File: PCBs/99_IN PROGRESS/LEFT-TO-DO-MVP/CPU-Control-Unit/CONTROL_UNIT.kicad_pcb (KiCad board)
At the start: 2 copper layers, 120.6 x 59.2 mm, 16 parts, among them U1 PLCC32_28_28C256, U10 74LS08, U11 74LS08, U12 74LS139, U13 74LS154, U14 74LS08, U15 74HC245, U16 74HC245, U2 74HC245, U3 74HC245, U4 PLCC32_28_28C256, U5 74LS139, U6 74LS154, U7 74LS154, U8 74LS04, U9 74LS08

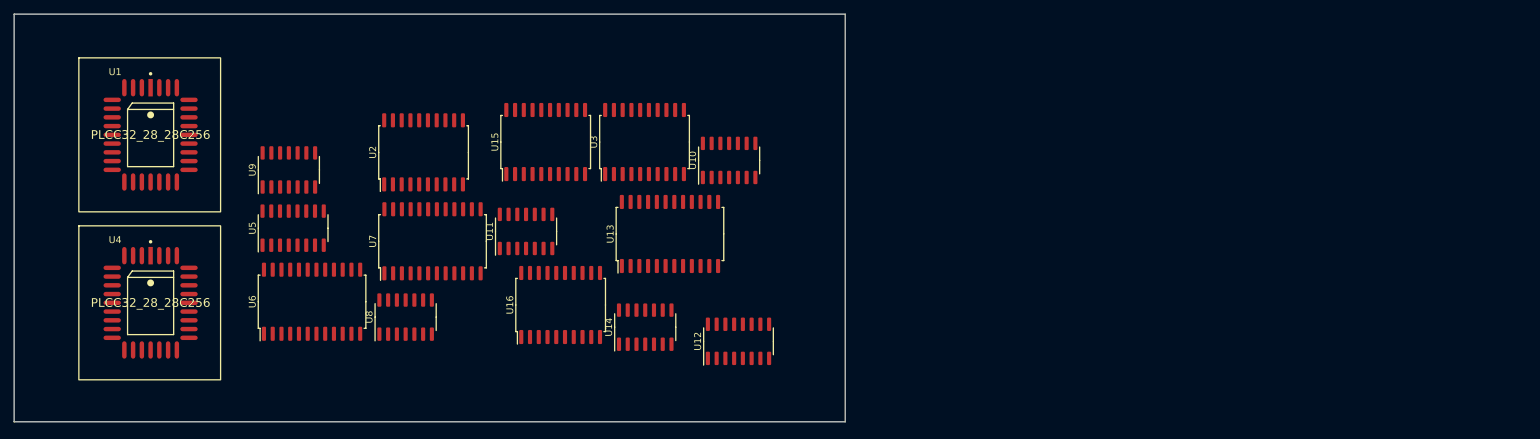
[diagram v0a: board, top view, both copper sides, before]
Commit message: saving
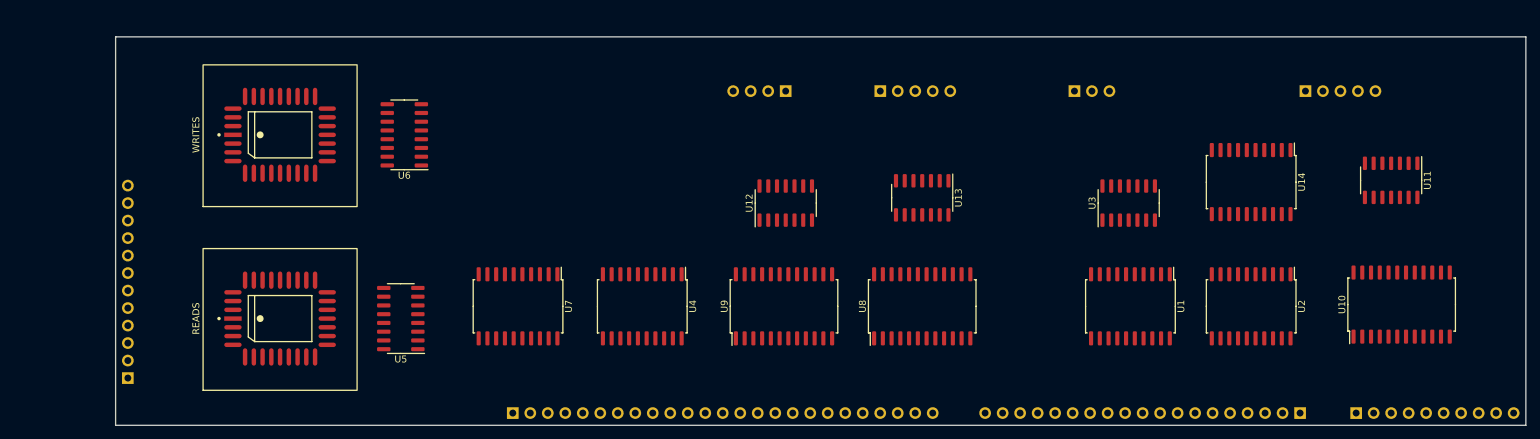
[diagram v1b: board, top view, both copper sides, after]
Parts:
- added J1: Conn_01x05, Connector_PinHeader_2.54mm:PinHeader_1x05_P2.54mm_Vertical, B.Cu at (224.3, 68.3)
- added J2: Conn_01x12, Connector_PinHeader_2.54mm:PinHeader_1x12_P2.54mm_Vertical, B.Cu at (53.3, 110.0)
- added J3: Conn_01x03, Connector_PinHeader_2.54mm:PinHeader_1x03_P2.54mm_Vertical, B.Cu at (190.8, 68.3)
- added J4: Conn_01x05, Connector_PinHeader_2.54mm:PinHeader_1x05_P2.54mm_Vertical, B.Cu at (162.6, 68.3)
- added J5: Conn_01x25, Connector_PinHeader_2.54mm:PinHeader_1x25_P2.54mm_Vertical, B.Cu at (109.2, 115.1)
- added J6: Conn_01x19, Connector_PinHeader_2.54mm:PinHeader_1x19_P2.54mm_Vertical, B.Cu at (223.5, 115.1)
- added J7: Conn_01x04, Connector_PinHeader_2.54mm:PinHeader_1x04_P2.54mm_Vertical, B.Cu at (148.8, 68.3)
- added J8: Conn_01x10, Connector_PinHeader_2.54mm:PinHeader_1x10_P2.54mm_Vertical, B.Cu at (231.6, 115.1)
- U1, U4: value PLCC32_28_28C256 -> 74HC245; footprint Stephenv6:PLCC-32-SOCKET-Microchip-32J-10_2001-B-IPC_A -> Package_SO:SOIC-20W_7.5x12.8mm_P1.27mm
- U10, U9: value 74LS08 -> 74LS154; footprint Package_SO:SOIC-14_3.9x8.7mm_P1.27mm -> Package_SO:SOIC-24W_7.5x15.4mm_P1.27mm
- U12: value 74LS139 -> 74LS08; footprint Package_SO:SOIC-16_3.9x9.9mm_P1.27mm -> Package_SO:SOIC-14_3.9x8.7mm_P1.27mm
- U13: value 74LS154 -> 74LS08; footprint Package_SO:SOIC-24W_7.5x15.4mm_P1.27mm -> Package_SO:SOIC-14_3.9x8.7mm_P1.27mm
- U14: value 74LS08 -> 74HC245; footprint Package_SO:SOIC-14_3.9x8.7mm_P1.27mm -> Package_SO:SOIC-20W_7.5x12.8mm_P1.27mm
- U15, U16: value 74HC245 -> PLCC32_28_28C256; footprint Package_SO:SOIC-20W_7.5x12.8mm_P1.27mm -> LIBRARY-8-bit-computer:Socket-PLCC-32
- U3: value 74HC245 -> 74LS08; footprint Package_SO:SOIC-20W_7.5x12.8mm_P1.27mm -> Package_SO:SOIC-14_3.9x8.7mm_P1.27mm
- U6: value 74LS154 -> 74LS138; footprint Package_SO:SOIC-24W_7.5x15.4mm_P1.27mm -> Package_SO:SOIC-16_3.9x9.9mm_P1.27mm
- U7: value 74LS154 -> 74HC245; footprint Package_SO:SOIC-24W_7.5x15.4mm_P1.27mm -> Package_SO:SOIC-20W_7.5x12.8mm_P1.27mm
- U8: value 74LS04 -> 74LS154; footprint Package_SO:SOIC-14_3.9x8.7mm_P1.27mm -> Package_SO:SOIC-24W_7.5x15.4mm_P1.27mm
- moved U1 144.4 mm to (198.9, 99.6), turned to -90 degrees
- moved U11 125.8 mm to (236.7, 81.3), turned to -90 degrees
- moved U2 122.2 mm to (216.4, 99.6), turned to -90 degrees
- moved U10 99.8 mm to (238.3, 99.3)
- moved U14 90.4 mm to (216.4, 81.5), turned to -90 degrees
- moved U8 75.0 mm to (168.7, 99.6)
- moved U9 74.6 mm to (148.6, 99.6)
- moved U4 71.4 mm to (128.0, 99.6), turned to -90 degrees
- moved U3 70.8 mm to (198.6, 84.6)
- moved U16 47.6 mm to (75.4, 74.7)
- moved U15 46.3 mm to (75.4, 101.3)
- moved U13 37.0 mm to (168.7, 83.8), turned to -90 degrees
- moved U6 27.7 mm to (93.5, 74.7), turned to 180 degrees
- moved U12 21.2 mm to (148.8, 84.6)
- moved U5 20.4 mm to (93.0, 101.3), turned to 180 degrees
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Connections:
- net ~{EN_WRITE_0} renamed ~{EN_READ_GPR}
- U1 pad 1: unconnected-(U1-Pad1) -> VCC
- U1 pad 10: STEP1 -> GND
- U1 pad 11: STEP0 -> unconnected-(U1-Pad11)
- U1 pad 13: WRITE0 -> unconnected-(U1-Pad13)
- U1 pad 14: WRITE1 -> unconnected-(U1-Pad14)
- U1 pad 15: WRITE2 -> unconnected-(U1-Pad15)
- U1 pad 16: GND -> GPR2
- U1 pad 17: unconnected-(U1-Pad17) -> GPR1
- U1 pad 18: WRITE3 -> GPR0
- U1 pad 19: WRITE4 -> ~{EN_WRITE_GPR}
- U1 pad 2: GND -> μ2_0
- U1 pad 20: WRITE5 -> VCC
- U1 pad 3: GND -> μ2_1
- U1 pad 4: INSTRUCTION3 -> μ2_2
- U1 pad 5: INSTRUCTION2 -> GND
- U1 pad 6: INSTRUCTION1 -> GND
- U1 pad 7: INSTRUCTION0 -> GND
- U1 pad 8: STEP3 -> GND
- U1 pad 9: STEP2 -> GND
- U10 pad 1: /~{WRITE_DATA} -> ~{OFFSET_LATCH}
- U10 pad 10: IRQ_REG_SEL -> unconnected-(U10-Pad10)
- U10 pad 11: ~{IO_WRITE} -> unconnected-(U10-Pad11)
- U10 pad 12: /~{WRITE_IO} -> GND
- U10 pad 13: /~{WRITE_IO_MEM} -> unconnected-(U10-Pad13)
- U10 pad 14: VCC -> unconnected-(U10-Pad14)
- U10 pad 2: /~{WRITE_STACK} -> ~{INDEX_LOAD}
- U10 pad 3: ~{MEM_WRITE} -> ~{INDEX_DEC}
- U10 pad 4: RESTORE_FLAGS -> ~{INDEX_INC}
- U10 pad 5: Net-(U10-Pad5) -> /~{WRITE_IPR}
- U10 pad 6: ~{LATCH_FLAGS} -> INT_REG_SEL
- U10 pad 7: GND -> /~{WRITE_IO}
- U10 pad 8: ~{IRQ_WRITE} -> /~{WRITE_IO_MEM}
- U10 pad 9: Net-(U10-Pad9) -> unconnected-(U10-Pad9)
- U11 pad 1: /~{READ_IO} -> /~{READ_CODE}
- U11 pad 10: ~{IRQ_WRITE} -> /~{WRITE_DATA}
- U11 pad 11: ~{IO_READ} -> ~{MEM_WRITE}
- U11 pad 12: /~{READ_IO} -> Net-(U11-Pad12)
- U11 pad 13: /~{READ_IO_MEM} -> /~{WRITE_STACK}
- U11 pad 2: /~{WRITE_IO} -> /~{READ_DATA}
- U11 pad 3: ~{IO_REQUEST} -> Net-(U11-Pad3)
- U11 pad 4: /~{READ_IO_MEM} -> Net-(U11-Pad3)
- U11 pad 5: /~{WRITE_IO_MEM} -> /~{READ_STACK}
- U11 pad 6: ~{MEM_REQUEST} -> ~{MEM_READ}
- U11 pad 8: ~{IRQ_EN} -> Net-(U11-Pad12)
- U11 pad 9: ~{IRQ_READ} -> /~{WRITE_CODE}
- U12 pad 1: GND -> /~{WRITE_IO_MEM}
- U12 pad 10: unconnected-(U12-Pad10) -> /~{WRITE_IO}
- U12 pad 11: unconnected-(U12-Pad11) -> ~{IO_MEM_REQUEST}
- U12 pad 12: unconnected-(U12-Pad12) -> /~{READ_IO_MEM}
- U12 pad 13: READ6 -> /~{WRITE_IO_MEM}
- U12 pad 14: READ7 -> VCC
- U12 pad 2: READ4 -> /~{WRITE_IO}
- U12 pad 3: READ5 -> ~{IO_WRITE}
- U12 pad 4: ~{EN_READ_0} -> /~{READ_IO}
- U12 pad 5: ~{EN_READ_1} -> /~{READ_IO_MEM}
- U12 pad 6: ~{EN_READ_2} -> ~{IO_READ}
- U12 pad 7: ~{EN_READ_3} -> GND
- U12 pad 8: GND -> ~{IO_REQUEST}
- U12 pad 9: unconnected-(U12-Pad9) -> /~{READ_IO}
- U13 pad 1: ~{LD_IR} -> FLAGS_RESTORE
- U13 pad 10: ~{NC_WRITE2_9} -> ~{INT_READ}
- U13 pad 11: ~{NC_WRITE2_10} -> unconnected-(U13-Pad11)
- U13 pad 13: ~{NC_WRITE2_11} -> GND
- U13 pad 14: ~{NC_WRITE2_12} -> VCC
- U13 pad 2: Net-(U13-Pad2) -> /~{RESTORE_FLAGS}
- U13 pad 3: ~{PC_DEC} -> ~{FLAGS_IN}
- U13 pad 4: ~{SP_LOAD} -> INT_REG_SEL
- U13 pad 5: ~{SP_DEC} -> /~{WRITE_IPR}
- U13 pad 6: ~{SP_INC} -> ~{INT_WRITE}
- U13 pad 7: ~{NC_WRITE2_6} -> GND
- U13 pad 8: ~{NC_WRITE2_7} -> ~{INT_EN}
- U13 pad 9: ~{NC_WRITE2_8} -> ~{INT_WRITE}
- U14 pad 1: ~{EN_READ_2} -> VCC
- U14 pad 12: GND -> unconnected-(U14-Pad12)
- U14 pad 13: GND -> unconnected-(U14-Pad13)
- U14 pad 14: VCC -> unconnected-(U14-Pad14)
- U14 pad 2: ~{EN_READ_3} -> μ2_0
- U14 pad 3: Net-(U14-Pad3) -> μ2_1
- U14 pad 4: ~{JCC_LD_PC_COND} -> μ2_2
- U14 pad 5: Net-(U13-Pad2) -> μ2_3
- U14 pad 6: ~{PC_LOAD} -> GND
- U14 pad 8: unconnected-(U14-Pad8) -> GND
- U15 pad 1: VCC -> unconnected-(U15-Pad1)
- U15 pad 10: GND -> STEP1
- U15 pad 11: unconnected-(U15-Pad11) -> STEP0
- U15 pad 13: ALU_FUNC_5 -> μ1_0
- U15 pad 14: ALU_FUNC_4 -> μ1_1
- U15 pad 15: ALU_FUNC_3 -> μ1_2
- U15 pad 16: ALU_FUNC_2 -> GND
- U15 pad 17: ALU_FUNC_1 -> unconnected-(U15-Pad17)
- U15 pad 18: ALU_FUNC_0 -> μ1_3
- U15 pad 19: Net-(U14-Pad3) -> μ1_4
- U15 pad 2: READ0 -> GND
- U15 pad 20: VCC -> μ1_5
- U15 pad 3: READ1 -> GND
- U15 pad 4: READ2 -> INSTRUCTION3
- U15 pad 5: READ3 -> INSTRUCTION2
- U15 pad 6: ~{EN_READ_2} -> INSTRUCTION1
- U15 pad 7: VCC -> INSTRUCTION0
- U15 pad 8: GND -> STEP3
- U15 pad 9: GND -> STEP2
- U16 pad 1: VCC -> unconnected-(U16-Pad1)
- U16 pad 10: GND -> STEP1
- U16 pad 11: unconnected-(U16-Pad11) -> STEP0
- U16 pad 13: unconnected-(U16-Pad13) -> μ2_0
- U16 pad 14: unconnected-(U16-Pad14) -> μ2_1
- U16 pad 15: JCC_ADR3 -> μ2_2
- U16 pad 16: JCC_ADR2 -> GND
- U16 pad 17: JCC_ADR1 -> unconnected-(U16-Pad17)
- U16 pad 18: JCC_ADR0 -> μ2_3
- U16 pad 19: ~{EN_WRITE_3} -> μ2_4
- U16 pad 2: WRITE0 -> GND
- U16 pad 20: VCC -> μ2_5
- U16 pad 3: WRITE1 -> GND
- U16 pad 4: WRITE2 -> INSTRUCTION3
- U16 pad 5: WRITE3 -> INSTRUCTION2
- U16 pad 6: GND -> INSTRUCTION1
- U16 pad 7: GND -> INSTRUCTION0
- U16 pad 8: GND -> STEP3
- U16 pad 9: GND -> STEP2
- U2 pad 15: unconnected-(U2-Pad15) -> GPR6
- U2 pad 16: GPR2 -> GPR5
- U2 pad 17: GPR1 -> GPR4
- U2 pad 18: GPR0 -> GPR3
- U2 pad 2: WRITE0 -> μ1_0
- U2 pad 3: WRITE1 -> μ1_1
- U2 pad 4: WRITE2 -> μ1_2
- U2 pad 5: GND -> μ1_3
- U3 pad 1: VCC -> ~{EN_ALU}
- U3 pad 10: GND -> /~{WRITE_DATA}
- U3 pad 11: unconnected-(U3-Pad11) -> ~{STACK_SEG_EN}
- U3 pad 12: unconnected-(U3-Pad12) -> /~{READ_STACK}
- U3 pad 13: unconnected-(U3-Pad13) -> /~{WRITE_STACK}
- U3 pad 14: unconnected-(U3-Pad14) -> VCC
- U3 pad 2: READ0 -> ~{EN_ALU_INVERT}
- U3 pad 3: READ1 -> Net-(U3-Pad3)
- U3 pad 4: READ2 -> /~{READ_CODE}
- U3 pad 5: READ3 -> /~{WRITE_CODE}
- U3 pad 6: GND -> ~{CODE_SEG_EN}
- U3 pad 8: GND -> ~{DATA_SEG_EN}
- U3 pad 9: GND -> /~{READ_DATA}
- U4 pad 1: unconnected-(U4-Pad1) -> VCC
- U4 pad 10: STEP1 -> GND
- U4 pad 11: STEP0 -> unconnected-(U4-Pad11)
- U4 pad 13: READ0 -> unconnected-(U4-Pad13)
- U4 pad 14: READ1 -> unconnected-(U4-Pad14)
- U4 pad 15: READ2 -> JCC_ADR3
- U4 pad 16: GND -> JCC_ADR2
- U4 pad 17: unconnected-(U4-Pad17) -> JCC_ADR1
- U4 pad 18: READ3 -> JCC_ADR0
- U4 pad 19: READ4 -> ~{EN_JCC}
- U4 pad 2: GND -> μ2_0
- U4 pad 20: READ5 -> VCC
- U4 pad 3: GND -> μ2_1
- U4 pad 4: INSTRUCTION3 -> μ2_2
- U4 pad 5: INSTRUCTION2 -> μ2_3
- U4 pad 6: INSTRUCTION1 -> GND
- U4 pad 7: INSTRUCTION0 -> GND
- U4 pad 8: STEP3 -> GND
- U4 pad 9: STEP2 -> GND
- U5 pad 10: ~{RESET_OP} -> ~{RESET_STEP}
- U5 pad 13: WRITE6 -> μ1_6
- U5 pad 14: WRITE7 -> μ1_7
- U5 pad 2: WRITE4 -> μ1_5
- U5 pad 3: WRITE5 -> μ1_4
- U5 pad 5: ~{EN_WRITE_1} -> ~{EN_ALU}
- U5 pad 6: ~{EN_WRITE_2} -> ~{EN_ALU_INVERT}
- U5 pad 7: ~{EN_WRITE_3} -> ~{EN_READ_GENERAL_CONTROL}
- U5 pad 9: ~{RESET} -> unconnected-(U5-Pad9)
- U6 pad 1: ~{LATCH_ACCUMULATOR} -> μ2_4
- U6 pad 10: Net-(U10-Pad5) -> ~{EN_WRITE_GENERAL_3}
- U6 pad 11: Net-(U10-Pad9) -> ~{DISPLACEMENT_LATCH}
- U6 pad 12: GND -> ~{EN_WRITE_GENERAL_2}
- U6 pad 13: IRQ_REG_SEL -> ~{EN_WRITE_GENERAL_1}
- U6 pad 14: /~{WRITE_IO} -> ~{EN_JCC}
- U6 pad 15: /~{WRITE_IO_MEM} -> ~{EN_WRITE_GPR}
- U6 pad 16: ~{NC_WRITE1_14} -> VCC
- U6 pad 2: ~{LATCH_B} -> μ2_5
- U6 pad 3: ~{MEM_LATCH_MAR} -> μ2_6
- U6 pad 4: ~{LATCH_CODE_SEG} -> GND
- U6 pad 5: ~{LATCH_DATA_SEG} -> GND
- U6 pad 6: ~{LATCH_STACK_SEG} -> VCC
- U6 pad 7: /~{WRITE_DATA} -> ~{EN_WRITE_GENERAL_5}
- U6 pad 8: /~{WRITE_STACK} -> GND
- U6 pad 9: RESTORE_FLAGS -> ~{EN_WRITE_GENERAL_4}
- U7 pad 1: ~{EN_CODE_SEG} -> VCC
- U7 pad 10: /~{READ_IO} -> GND
- U7 pad 11: /~{READ_IO_MEM} -> unconnected-(U7-Pad11)
- U7 pad 12: GND -> unconnected-(U7-Pad12)
- U7 pad 13: ~{IRQ_READ} -> ALU_FUNC_5
- U7 pad 14: ~{NC_READ1_12} -> ALU_FUNC_4
- U7 pad 15: ~{NC_READ1_13} -> ALU_FUNC_3
- U7 pad 16: ~{NC_READ1_14} -> ALU_FUNC_2
- U7 pad 17: ~{NC_READ1_15} -> ALU_FUNC_1
- U7 pad 18: ~{EN_READ_1} -> ALU_FUNC_0
- U7 pad 19: ~{EN_READ_1} -> Net-(U3-Pad3)
- U7 pad 2: Net-(U7-Pad2) -> μ1_0
- U7 pad 20: READ3 -> VCC
- U7 pad 3: Net-(U7-Pad3) -> μ1_1
- U7 pad 4: ~{ASSERT_CODE_SEG} -> μ1_2
- U7 pad 5: ~{ASSERT_DATA_SEG} -> μ1_3
- U7 pad 6: ~{ASSERT_STACK_SEG} -> ~{EN_ALU}
- U7 pad 7: ~{ASSERT_PC} -> VCC
- U7 pad 8: ~{ASSERT_SP} -> GND
- U7 pad 9: ~{ASSERT_FLAGS} -> GND
- U8 pad 1: ~{RESET} -> /~{WRITE_CODE}
- U8 pad 10: unconnected-(U8-Pad10) -> ~{SP_DEC}
- U8 pad 11: GND -> ~{SP_LOAD}
- U8 pad 12: unconnected-(U8-Pad12) -> GND
- U8 pad 13: GND -> FLAGS_RESTORE
- U8 pad 14: VCC -> /~{RESTORE_FLAGS}
- U8 pad 2: RESET -> /~{WRITE_DATA}
- U8 pad 3: GND -> /~{WRITE_STACK}
- U8 pad 4: unconnected-(U8-Pad4) -> ~{MEM_LATCH_MAR}
- U8 pad 5: GND -> ~{CODE_SEG_IN}
- U8 pad 6: unconnected-(U8-Pad6) -> ~{DATA_SEG_IN}
- U8 pad 7: GND -> ~{STACK_SEG_IN}
- U8 pad 8: unconnected-(U8-Pad8) -> ~{PC_DEC}
- U8 pad 9: GND -> ~{SP_INC}
- U9 pad 1: ~{EN_CODE_SEG} -> /~{READ_CODE}
- U9 pad 10: /~{WRITE_DATA} -> ~{SP_OUT}
- U9 pad 11: ~{EN_STACK_SEG} -> /~{READ_IO}
- U9 pad 12: Net-(U7-Pad3) -> GND
- U9 pad 13: /~{WRITE_STACK} -> /~{READ_IO_MEM}
- U9 pad 14: VCC -> ~{DISPLACEMENT_OUT}
- U9 pad 2: Net-(U7-Pad2) -> /~{READ_DATA}
- U9 pad 3: Net-(U9-Pad3) -> /~{READ_STACK}
- U9 pad 4: Net-(U9-Pad3) -> ~{STACK_SEG_OUT}
- U9 pad 5: Net-(U7-Pad3) -> ~{DATA_SEG_OUT}
- U9 pad 6: ~{MEM_READ} -> ~{CODE_SEG_OUT}
- U9 pad 7: GND -> ~{INT_READ}
- U9 pad 8: ~{EN_DATA_SEG} -> ~{FLAGS_OUT}
- U9 pad 9: Net-(U7-Pad2) -> ~{PC_OUT}
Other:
- board size 120.6 x 59.2 mm -> 204.7 x 56.4 mm
